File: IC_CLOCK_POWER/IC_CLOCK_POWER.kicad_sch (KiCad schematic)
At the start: 24 parts, among them J1 Conn_01x02_Pin, J2 Conn_01x04_Pin, U1 LM317T, U2 L7805

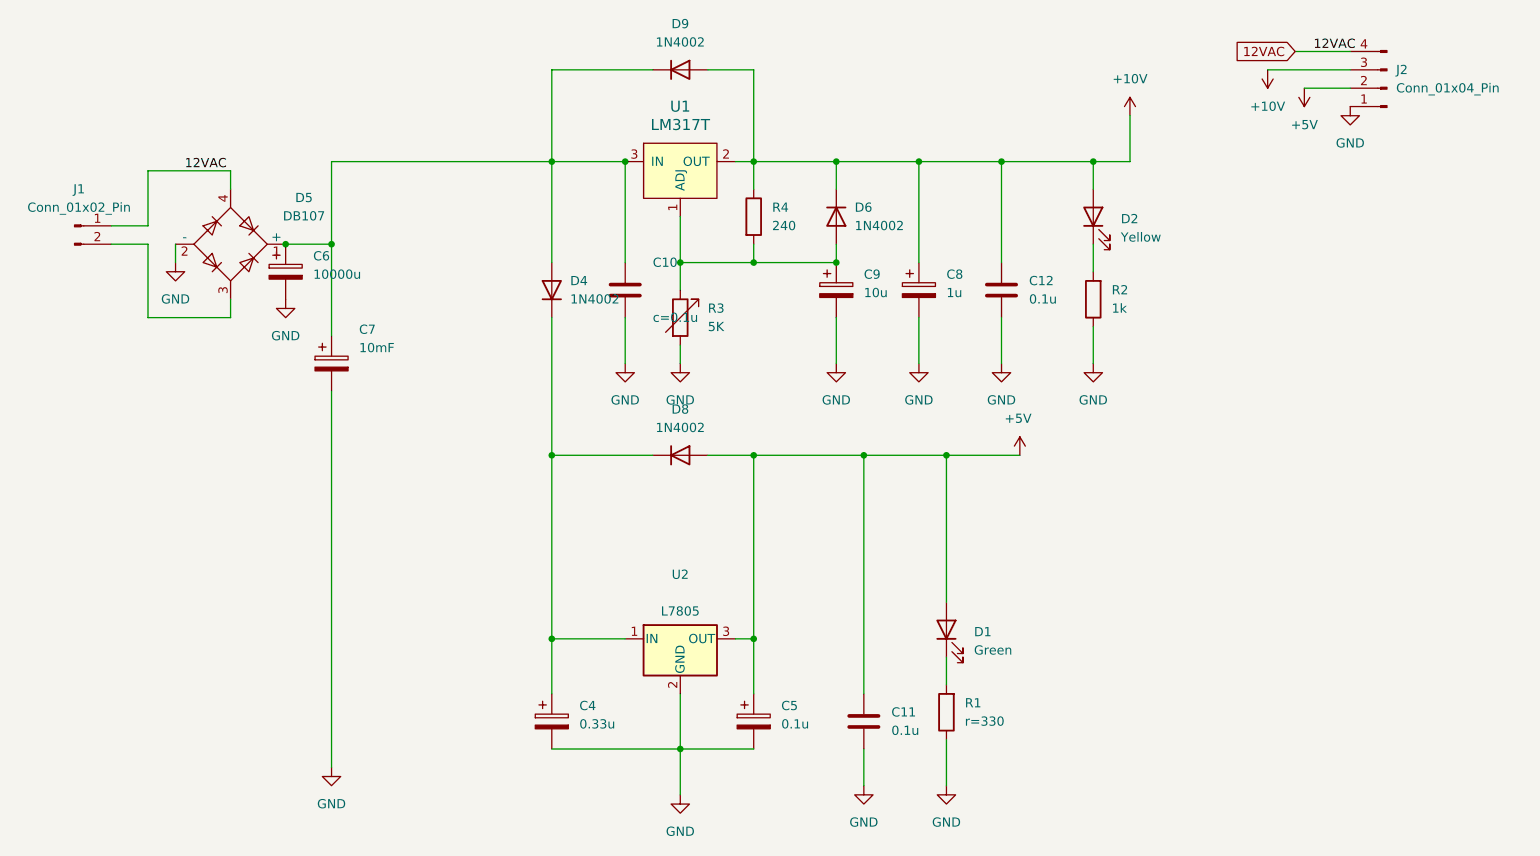
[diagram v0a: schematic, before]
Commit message: Fixing schematic ..
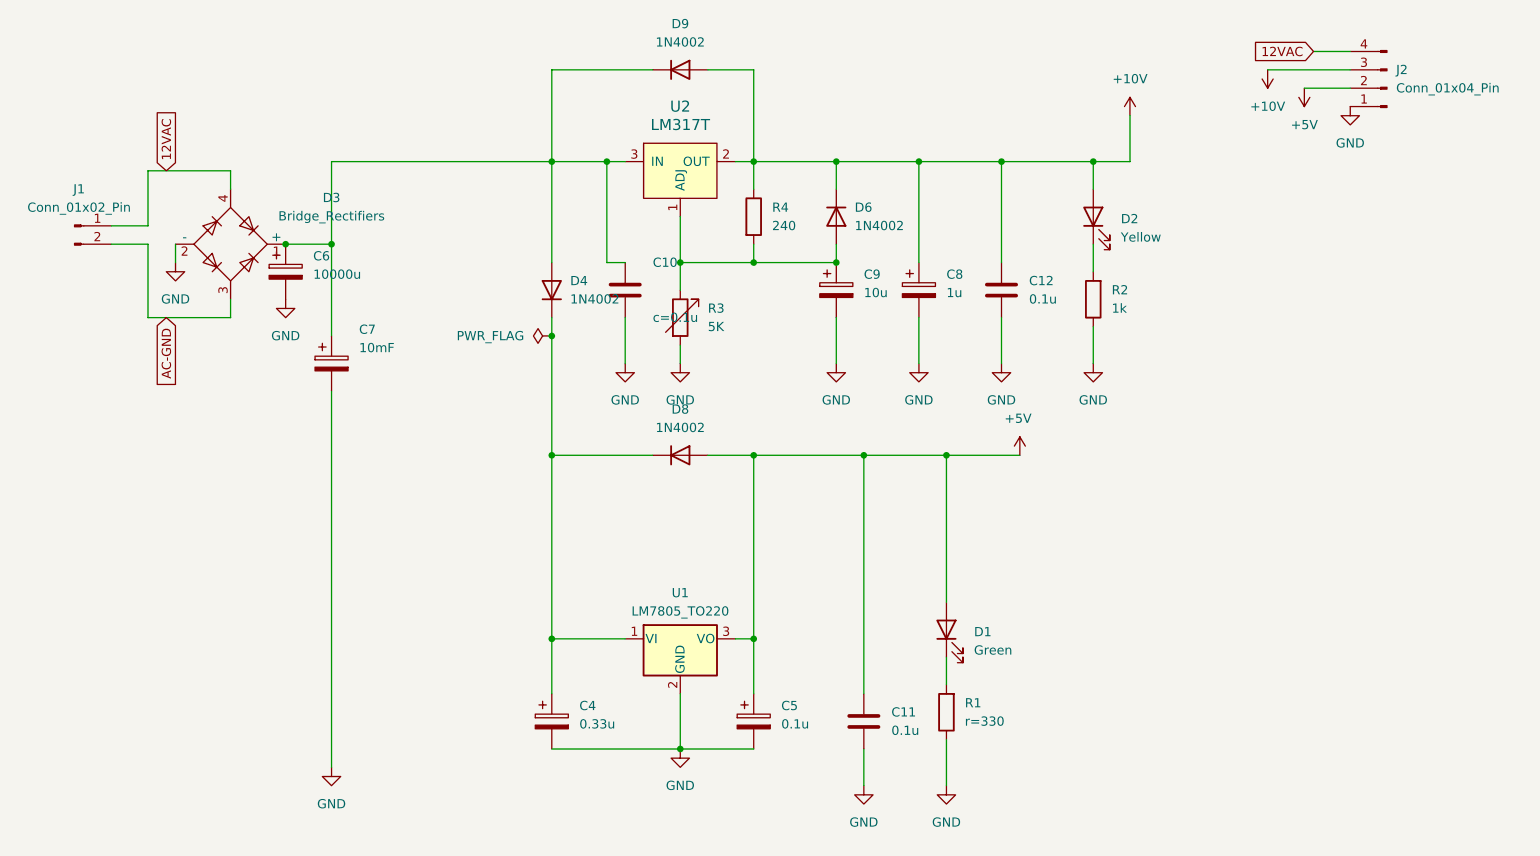
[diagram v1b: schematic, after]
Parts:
- removed D5: DB107, IC_CLOCK:Bridge_Rectifier_4EDIP, symbol IC_CLOCK:Bridge_Rectifiers
- removed U1: LM317T, Package_TO_SOT_THT:TO-220F-3_HEATSINK_Vertical, symbol dk_PMIC-Voltage-Regulators-Linear:LM317T
- removed U2: L7805, Package_TO_SOT_THT:TO-220F-3_HEATSINK_Vertical, symbol Regulator_Linear:L7805
- added D3: Bridge_Rectifiers, IC_CLOCK:Bridge_Rectifier_4EDIP, symbol IC_CLOCK:Bridge_Rectifiers
- added U1: LM7805_TO220, Package_TO_SOT_THT:TO-220-3_Vertical, symbol Regulator_Linear:LM7805_TO220
- added U2: LM317T, digikey-footprints:TO-220-3, symbol dk_PMIC-Voltage-Regulators-Linear:LM317T
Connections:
- net +10V: now also U2.2 (OUT)
- net +5V: now also U1.3 (VO)
- net 12VAC: now also D3.4
- net GND: now also D3.2 (-), U1.2 (GND)
- net at C9.1, D6.2 (A), R3.1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: now also U2.1 (ADJ)
- net AC-GND: now reaches J1.2 (Pin_2)
- net AC-GND: now also D3.3
- net at C4.1, D4.1 (K), D8.1 (K): now also U1.1 (VI)
- net at C10.2, C6.1, C7.1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: now also D3.1 (+), U2.3 (IN)
